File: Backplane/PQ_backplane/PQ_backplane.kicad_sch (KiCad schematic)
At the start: 13 parts, among them J1 M55-6002642R, J2 FTSH-107-01-L-DV-K-A, J3 M55-6002642R, J4 M55-6001242R, J5 USB4110-GF-A, J6 M55-7104042R, U4 FUSB302BMPX

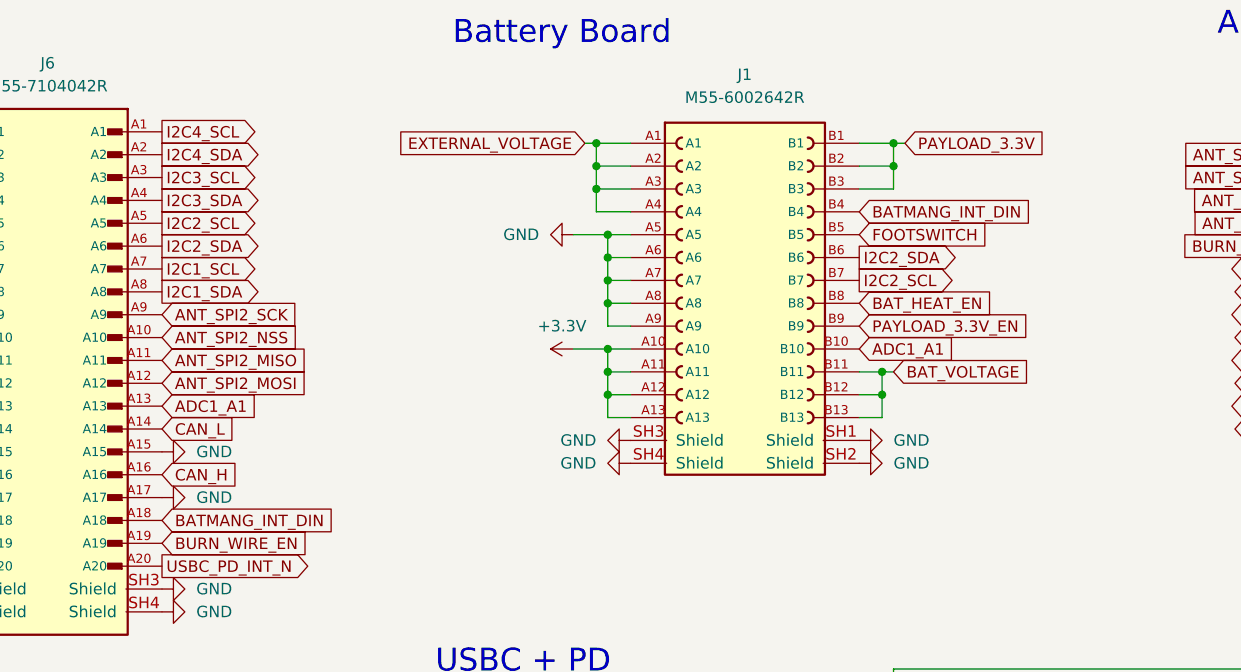
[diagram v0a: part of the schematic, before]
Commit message: Board sizes for FC and routing. slight Backplane changes
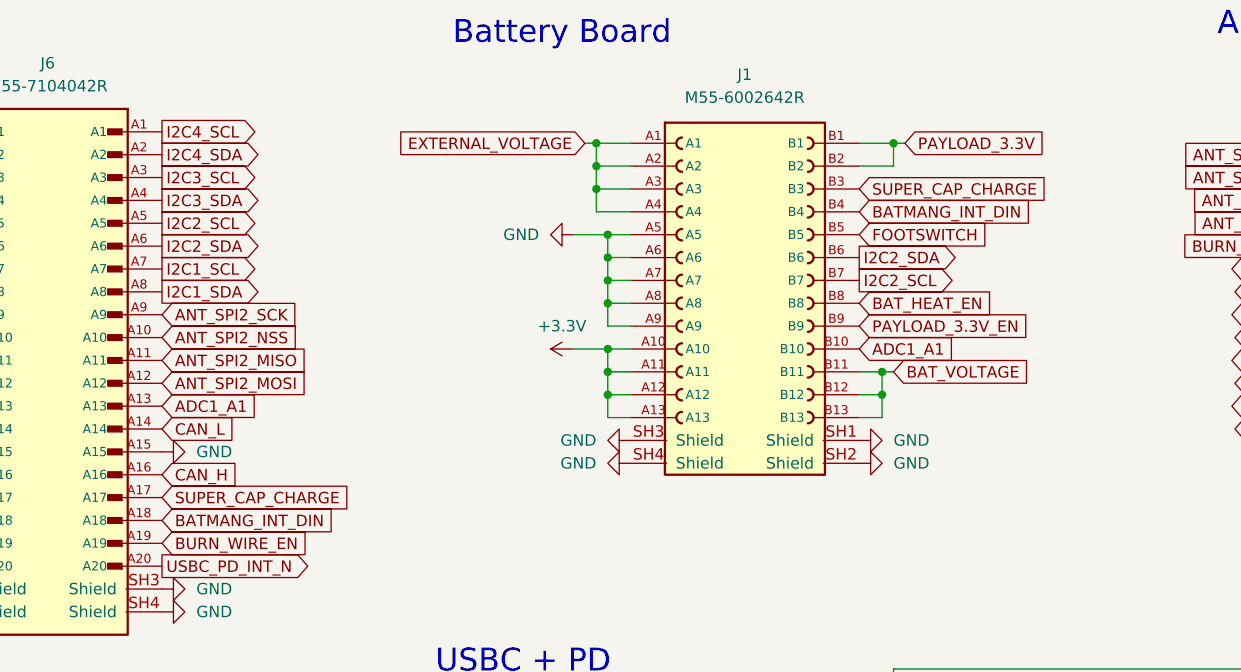
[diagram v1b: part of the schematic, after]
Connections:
- net GND: no longer J6.A17
- net PAYLOAD_3.3V: no longer J1.B3
- new net SUPER_CAP_CHARGE: J1.B3, J6.A17
